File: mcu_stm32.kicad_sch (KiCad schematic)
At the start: 23 parts, among them J1 Boot_Sel, J2 Debug, SW1 RESET, U1 STM32F103C8Tx, Y1 8mHz, Y2 32.768kHz

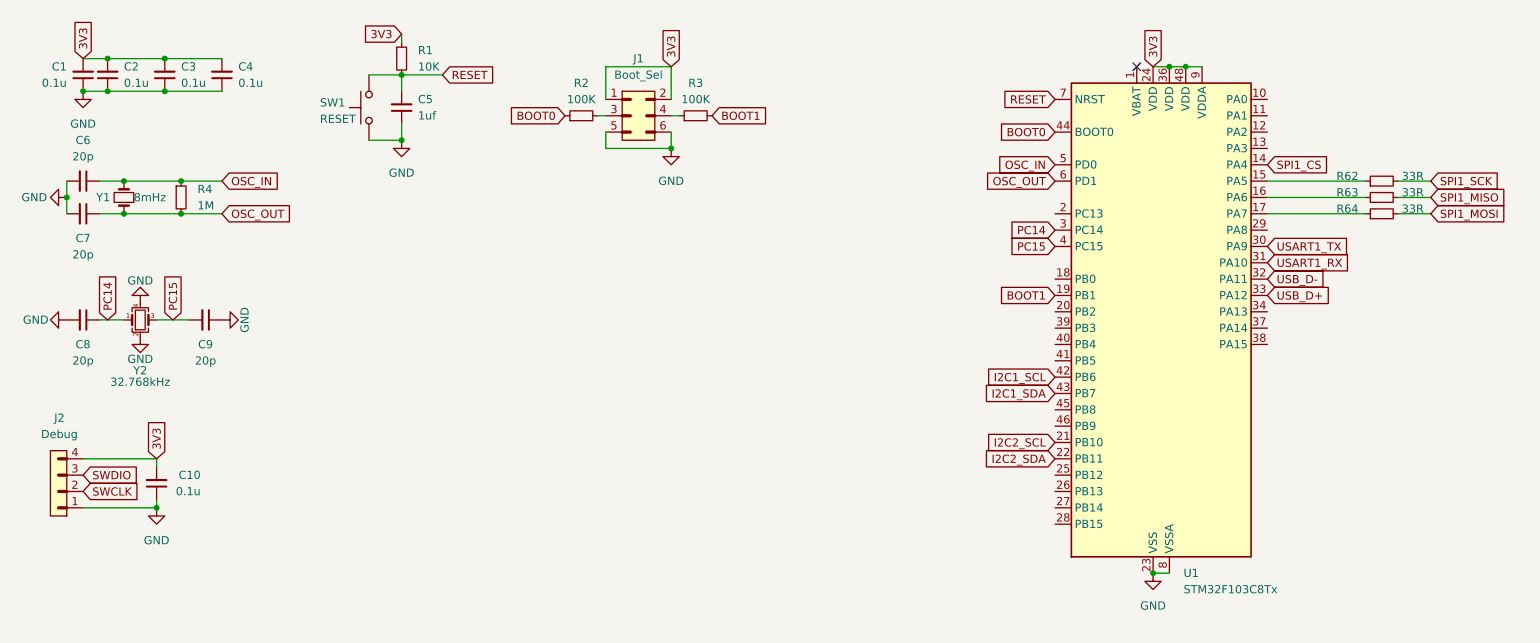
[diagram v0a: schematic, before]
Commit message: Visual Improvements
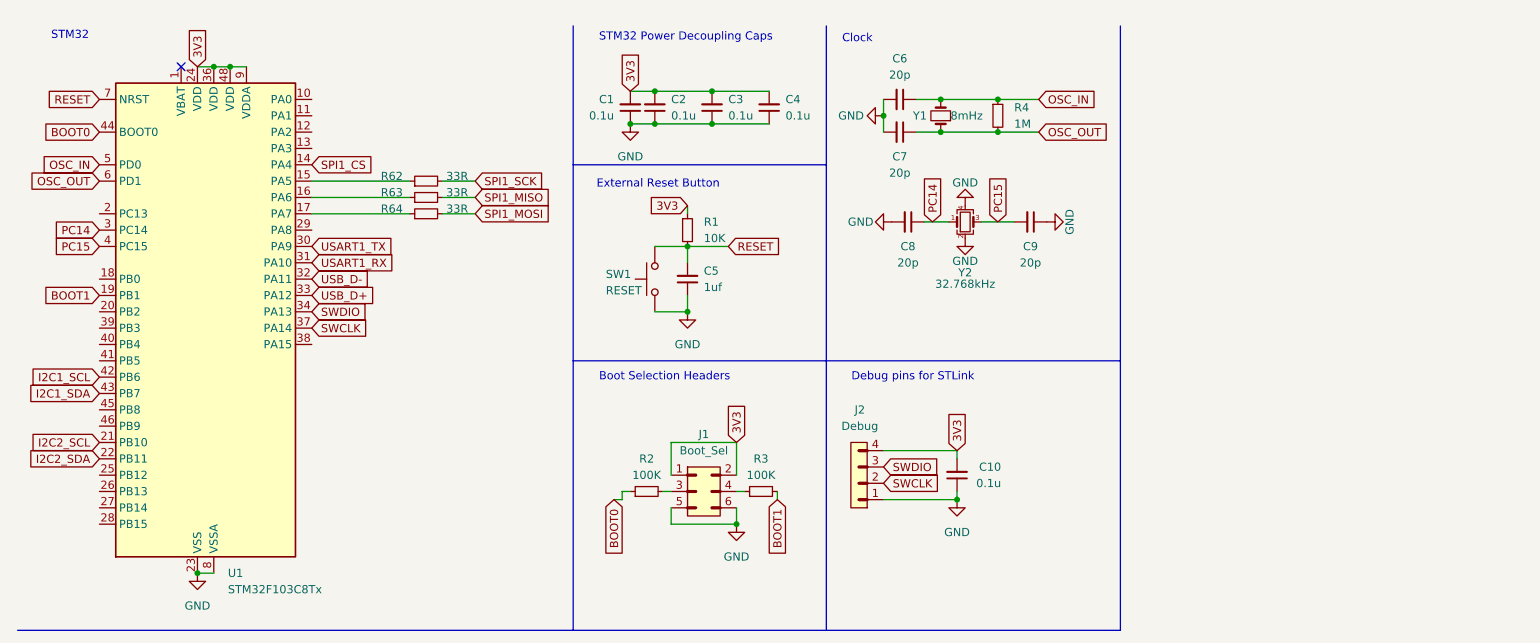
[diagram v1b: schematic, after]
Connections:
- net SWCLK: now also U1.37 (PA14)
- net SWDIO: now also U1.34 (PA13)
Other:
- note added: "Boot Selection Headers"
- note added: "Clock"
- note added: "Debug pins for STLink"
- note added: "External Reset Button"
- note added: "STM32"
- note added: "STM32 Power Decoupling Caps"
- moved on the sheet: C1, C10, C2, C3, C4, C5, C6, C7, C8, C9, J1, J2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

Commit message: schematic finished
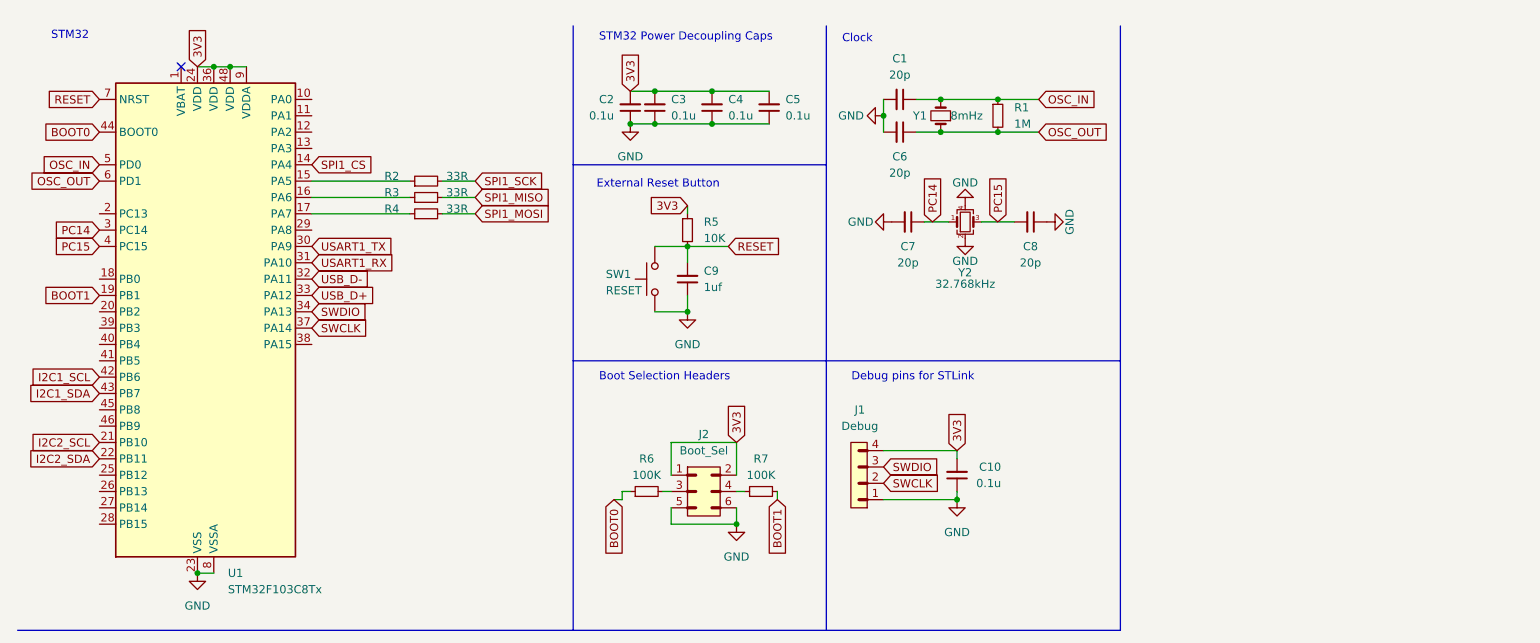
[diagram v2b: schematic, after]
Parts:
- SW1: footprint Button_Switch_SMD:SW_SPST_CK_KMS2xxGP -> Button_Switch_SMD:SW_SPST_B3U-1000P
- Y1: footprint (none) -> Crystal:Crystal_HC49-U_Vertical
- Y2: footprint (none) -> Crystal:Crystal_SMD_2016-4Pin_2.0x1.6mm
- renumbered C6 to C1, C1 to C2, C2 to C3, C3 to C4, C4 to C5, C7 to C6, C8 to C7, C9 to C8, C5 to C9, J2 to J1, J1 to J2, R4 to R1, R62 to R2, R63 to R3, R64 to R4, R1 to R5, R2 to R6, R3 to R7
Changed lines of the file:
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@@
 		(dnp no)
 		(fields_autoplaced yes)
-		(property "Reference" "C4"
+		(property "Reference" "C5"
 			(at 132.08 25.3935 0)
 			(effects
@@
 			(project "controllerForVehicle"
 				(path "/f177fb06-71dc-4865-9331-a828b12c2bf7/3df2cc68-9e37-4ed2-a8f2-6c459eac7ab6"
-					(reference "C4")
+					(reference "C5")
 					(unit 1)
 				)
@@
 			)
 		)
-		(property "Footprint" ""
+		(property "Footprint" "Crystal:Crystal_HC49-U_Vertical"
 			(at 156.21 27.94 0)
 			(effects
@@
 		(on_board yes)
 		(dnp no)
-		(property "Reference" "#PWR08"
+		(property "Reference" "#PWR06"
 			(at 160.02 53.34 0)
 			(effects
@@
 			(project "controllerForVehicle"
 				(path "/f177fb06-71dc-4865-9331-a828b12c2bf7/3df2cc68-9e37-4ed2-a8f2-6c459eac7ab6"
-					(reference "#PWR08")
+					(reference "#PWR06")
 					(unit 1)
 				)
@@
 		(on_board yes)
 		(dnp no)
-		(property "Reference" "R62"
+		(property "Reference" "R2"
 			(at 70.866 37.338 90)
 			(effects
@@
 			(project "controllerForVehicle"
 				(path "/f177fb06-71dc-4865-9331-a828b12c2bf7/3df2cc68-9e37-4ed2-a8f2-6c459eac7ab6"
-					(reference "R62")
+					(reference "R2")
 					(unit 1)
 				)
@@
 		(dnp no)
 		(fields_autoplaced yes)
-		(property "Reference" "R2"
+		(property "Reference" "R6"
 			(at 110.49 81.28 90)
 			(effects
@@
 			(project "controllerForVehicle"
 				(path "/f177fb06-71dc-4865-9331-a828b12c2bf7/3df2cc68-9e37-4ed2-a8f2-6c459eac7ab6"
-					(reference "R2")
+					(reference "R6")
 					(unit 1)
 				)
@@
 		(on_board yes)
 		(dnp no)
-		(property "Reference" "R63"
+		(property "Reference" "R3"
 			(at 70.866 39.878 90)
 			(effects
@@
 			(project "controllerForVehicle"
 				(path "/f177fb06-71dc-4865-9331-a828b12c2bf7/3df2cc68-9e37-4ed2-a8f2-6c459eac7ab6"
-					(reference "R63")
+					(reference "R3")
 					(unit 1)
 				)
@@
 		(on_board yes)
 		(dnp no)
-		(property "Reference" "#PWR04"
+		(property "Reference" "#PWR01"
 			(at 140.97 27.94 0)
 			(effects
@@
 			(project "controllerForVehicle"
 				(path "/f177fb06-71dc-4865-9331-a828b12c2bf7/3df2cc68-9e37-4ed2-a8f2-6c459eac7ab6"
-					(reference "#PWR04")
+					(reference "#PWR01")
 					(unit 1)
 				)
@@
 		(dnp no)
 		(fields_autoplaced yes)
-		(property "Reference" "C1"
+		(property "Reference" "C2"
 			(at 105.41 25.3935 0)
 			(effects
@@
 			(project "controllerForVehicle"
 				(path "/f177fb06-71dc-4865-9331-a828b12c2bf7/3df2cc68-9e37-4ed2-a8f2-6c459eac7ab6"
-					(reference "C1")
+					(reference "C2")
 					(unit 1)
 				)
@@
 		(on_board yes)
 		(dnp no)
-		(property "Reference" "R64"
+		(property "Reference" "R4"
 			(at 70.866 42.418 90)
 			(effects
@@
 			(project "controllerForVehicle"
 				(path "/f177fb06-71dc-4865-9331-a828b12c2bf7/3df2cc68-9e37-4ed2-a8f2-6c459eac7ab6"
-					(reference "R64")
+					(reference "R4")
 					(unit 1)
 				)
@@
 			)
 		)
-		(property "Footprint" "Button_Switch_SMD:SW_SPST_CK_KMS2xxGP"
+		(property "Footprint" "Button_Switch_SMD:SW_SPST_B3U-1000P"
 			(at 106.68 53.34 0)
 			(effects
@@
 		(on_board yes)
 		(dnp no)
-		(property "Reference" "#PWR07"
+		(property "Reference" "#PWR05"
 			(at 179.07 44.45 0)
 			(effects
@@
 			(project "controllerForVehicle"
 				(path "/f177fb06-71dc-4865-9331-a828b12c2bf7/3df2cc68-9e37-4ed2-a8f2-6c459eac7ab6"
-					(reference "#PWR07")
+					(reference "#PWR05")
 					(unit 1)
 				)
@@
 		(dnp no)
 		(fields_autoplaced yes)
-		(property "Reference" "J2"
+		(property "Reference" "J1"
 			(at 143.635 73.66 0)
 			(effects
@@
 			(project ""
 				(path "/f177fb06-71dc-4865-9331-a828b12c2bf7/3df2cc68-9e37-4ed2-a8f2-6c459eac7ab6"
-					(reference "J2")
+					(reference "J1")
 					(unit 1)
 				)
@@
 		(dnp no)
 		(fields_autoplaced yes)
-		(property "Reference" "#PWR03"
+		(property "Reference" "#PWR09"
 			(at 124.46 97.79 0)
 			(effects
@@
 			(project "controllerForVehicle"
 				(path "/f177fb06-71dc-4865-9331-a828b12c2bf7/3df2cc68-9e37-4ed2-a8f2-6c459eac7ab6"
-					(reference "#PWR03")
+					(reference "#PWR09")
 					(unit 1)
 				)
@@
 		(dnp no)
 		(fields_autoplaced yes)
-		(property "Reference" "#PWR02"
+		(property "Reference" "#PWR07"
 			(at 116.84 64.77 0)
 			(effects
@@
 			(project "controllerForVehicle"
 				(path "/f177fb06-71dc-4865-9331-a828b12c2bf7/3df2cc68-9e37-4ed2-a8f2-6c459eac7ab6"
-					(reference "#PWR02")
+					(reference "#PWR07")
 					(unit 1)
 				)
@@
 		(dnp no)
 		(fields_autoplaced yes)
-		(property "Reference" "J1"
+		(property "Reference" "J2"
 			(at 119.38 77.47 0)
 			(effects
@@
 			(project ""
 				(path "/f177fb06-71dc-4865-9331-a828b12c2bf7/3df2cc68-9e37-4ed2-a8f2-6c459eac7ab6"
-					(reference "J1")
+					(reference "J2")
 					(unit 1)
 				)
@@
 		(dnp no)
 		(fields_autoplaced yes)
-		(property "Reference" "C7"
+		(property "Reference" "C6"
 			(at 149.8536 34.29 90)
 			(effects
@@
 			(project "controllerForVehicle"
 				(path "/f177fb06-71dc-4865-9331-a828b12c2bf7/3df2cc68-9e37-4ed2-a8f2-6c459eac7ab6"
-					(reference "C7")
+					(reference "C6")
 					(unit 1)
 				)
@@
 		(dnp no)
 		(fields_autoplaced yes)
-		(property "Reference" "C3"
+		(property "Reference" "C4"
 			(at 123.19 25.3935 0)
 			(effects
@@
 			(project "controllerForVehicle"
 				(path "/f177fb06-71dc-4865-9331-a828b12c2bf7/3df2cc68-9e37-4ed2-a8f2-6c459eac7ab6"
-					(reference "C3")
+					(reference "C4")
 					(unit 1)
 				)
@@
 		(on_board yes)
 		(dnp no)
-		(property "Reference" "#PWR06"
+		(property "Reference" "#PWR04"
 			(at 142.24 44.45 0)
 			(effects
@@
 			(project "controllerForVehicle"
 				(path "/f177fb06-71dc-4865-9331-a828b12c2bf7/3df2cc68-9e37-4ed2-a8f2-6c459eac7ab6"
-					(reference "#PWR06")
+					(reference "#PWR04")
 					(unit 1)
 				)
@@
 		(dnp no)
 		(fields_autoplaced yes)
-		(property "Reference" "#PWR09"
+		(property "Reference" "#PWR08"
 			(at 158.75 93.98 0)
 			(effects
@@
 			(project "controllerForVehicle"
 				(path "/f177fb06-71dc-4865-9331-a828b12c2bf7/3df2cc68-9e37-4ed2-a8f2-6c459eac7ab6"
-					(reference "#PWR09")
+					(reference "#PWR08")
 					(unit 1)
 				)
@@
 		(dnp no)
 		(fields_autoplaced yes)
-		(property "Reference" "C5"
+		(property "Reference" "C9"
 			(at 119.38 52.0635 0)
 			(effects
@@
 			(project "controllerForVehicle"
 				(path "/f177fb06-71dc-4865-9331-a828b12c2bf7/3df2cc68-9e37-4ed2-a8f2-6c459eac7ab6"
-					(reference "C5")
+					(reference "C9")
 					(unit 1)
 				)
@@
 			)
 		)
-		(property "Footprint" ""
+		(property "Footprint" "Crystal:Crystal_SMD_2016-4Pin_2.0x1.6mm"
 			(at 160.02 44.45 0)
 			(effects
@@
 		(dnp no)
 		(fields_autoplaced yes)
-		(property "Reference" "R1"
+		(property "Reference" "R5"
 			(at 119.38 44.4499 0)
 			(effects
@@
 			(project "controllerForVehicle"
 				(path "/f177fb06-71dc-4865-9331-a828b12c2bf7/3df2cc68-9e37-4ed2-a8f2-6c459eac7ab6"
-					(reference "R1")
+					(reference "R5")
 					(unit 1)
 				)
@@
 		(dnp no)
 		(fields_autoplaced yes)
-		(property "Reference" "#PWR01"
+		(property "Reference" "#PWR02"
 			(at 107.95 35.56 0)
 			(effects
@@
 			(project "controllerForVehicle"
 				(path "/f177fb06-71dc-4865-9331-a828b12c2bf7/3df2cc68-9e37-4ed2-a8f2-6c459eac7ab6"
-					(reference "#PWR01")
+					(reference "#PWR02")
 					(unit 1)
 				)
@@
 		(dnp no)
 		(fields_autoplaced yes)
-		(property "Reference" "R4"
+		(property "Reference" "R1"
 			(at 167.64 26.6699 0)
 			(effects
@@
 			(project "controllerForVehicle"
 				(path "/f177fb06-71dc-4865-9331-a828b12c2bf7/3df2cc68-9e37-4ed2-a8f2-6c459eac7ab6"
-					(reference "R4")
+					(reference "R1")
 					(unit 1)
 				)
@@
 		(dnp no)
 		(fields_autoplaced yes)
-		(property "Reference" "C9"
+		(property "Reference" "C8"
 			(at 170.1736 48.26 90)
 			(effects
@@
 			(project "controllerForVehicle"
 				(path "/f177fb06-71dc-4865-9331-a828b12c2bf7/3df2cc68-9e37-4ed2-a8f2-6c459eac7ab6"
-					(reference "C9")
+					(reference "C8")
 					(unit 1)
 				)
@@
 		(dnp no)
 		(fields_autoplaced yes)
-		(property "Reference" "C6"
+		(property "Reference" "C1"
 			(at 149.8536 19.05 90)
 			(effects
@@
 			(project "controllerForVehicle"
 				(path "/f177fb06-71dc-4865-9331-a828b12c2bf7/3df2cc68-9e37-4ed2-a8f2-6c459eac7ab6"
-					(reference "C6")
+					(reference "C1")
 					(unit 1)
 				)
@@
 		(dnp no)
 		(fields_autoplaced yes)
-		(property "Reference" "R3"
+		(property "Reference" "R7"
 			(at 128.27 81.28 90)
 			(effects
@@
 			(project "controllerForVehicle"
 				(path "/f177fb06-71dc-4865-9331-a828b12c2bf7/3df2cc68-9e37-4ed2-a8f2-6c459eac7ab6"
-					(reference "R3")
+					(reference "R7")
 					(unit 1)
 				)
@@
 		(dnp no)
 		(fields_autoplaced yes)
-		(property "Reference" "C2"
+		(property "Reference" "C3"
 			(at 114.3 25.3935 0)
 			(effects
@@
 			(project "controllerForVehicle"
 				(path "/f177fb06-71dc-4865-9331-a828b12c2bf7/3df2cc68-9e37-4ed2-a8f2-6c459eac7ab6"
-					(reference "C2")
+					(reference "C3")
 					(unit 1)
 				)
@@
 		(on_board yes)
 		(dnp no)
-		(property "Reference" "#PWR05"
+		(property "Reference" "#PWR03"
 			(at 160.02 35.56 0)
 			(effects
@@
 			(project "controllerForVehicle"
 				(path "/f177fb06-71dc-4865-9331-a828b12c2bf7/3df2cc68-9e37-4ed2-a8f2-6c459eac7ab6"
-					(reference "#PWR05")
+					(reference "#PWR03")
 					(unit 1)
 				)
@@
 		(dnp no)
 		(fields_autoplaced yes)
-		(property "Reference" "C8"
+		(property "Reference" "C7"
 			(at 151.1236 48.26 90)
 			(effects
@@
 			(project "controllerForVehicle"
 				(path "/f177fb06-71dc-4865-9331-a828b12c2bf7/3df2cc68-9e37-4ed2-a8f2-6c459eac7ab6"
-					(reference "C8")
-					(unit 1)
-				)
+					(reference "C7")
+					(unit 1)
+				)
